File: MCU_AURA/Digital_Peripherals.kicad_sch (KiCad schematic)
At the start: 20 parts, among them J1 TF-CARD_H1.8, Q300 BSS138, Q301 BSS138, Q302 BSS138, U300 ICM-20948, U301 BMP280

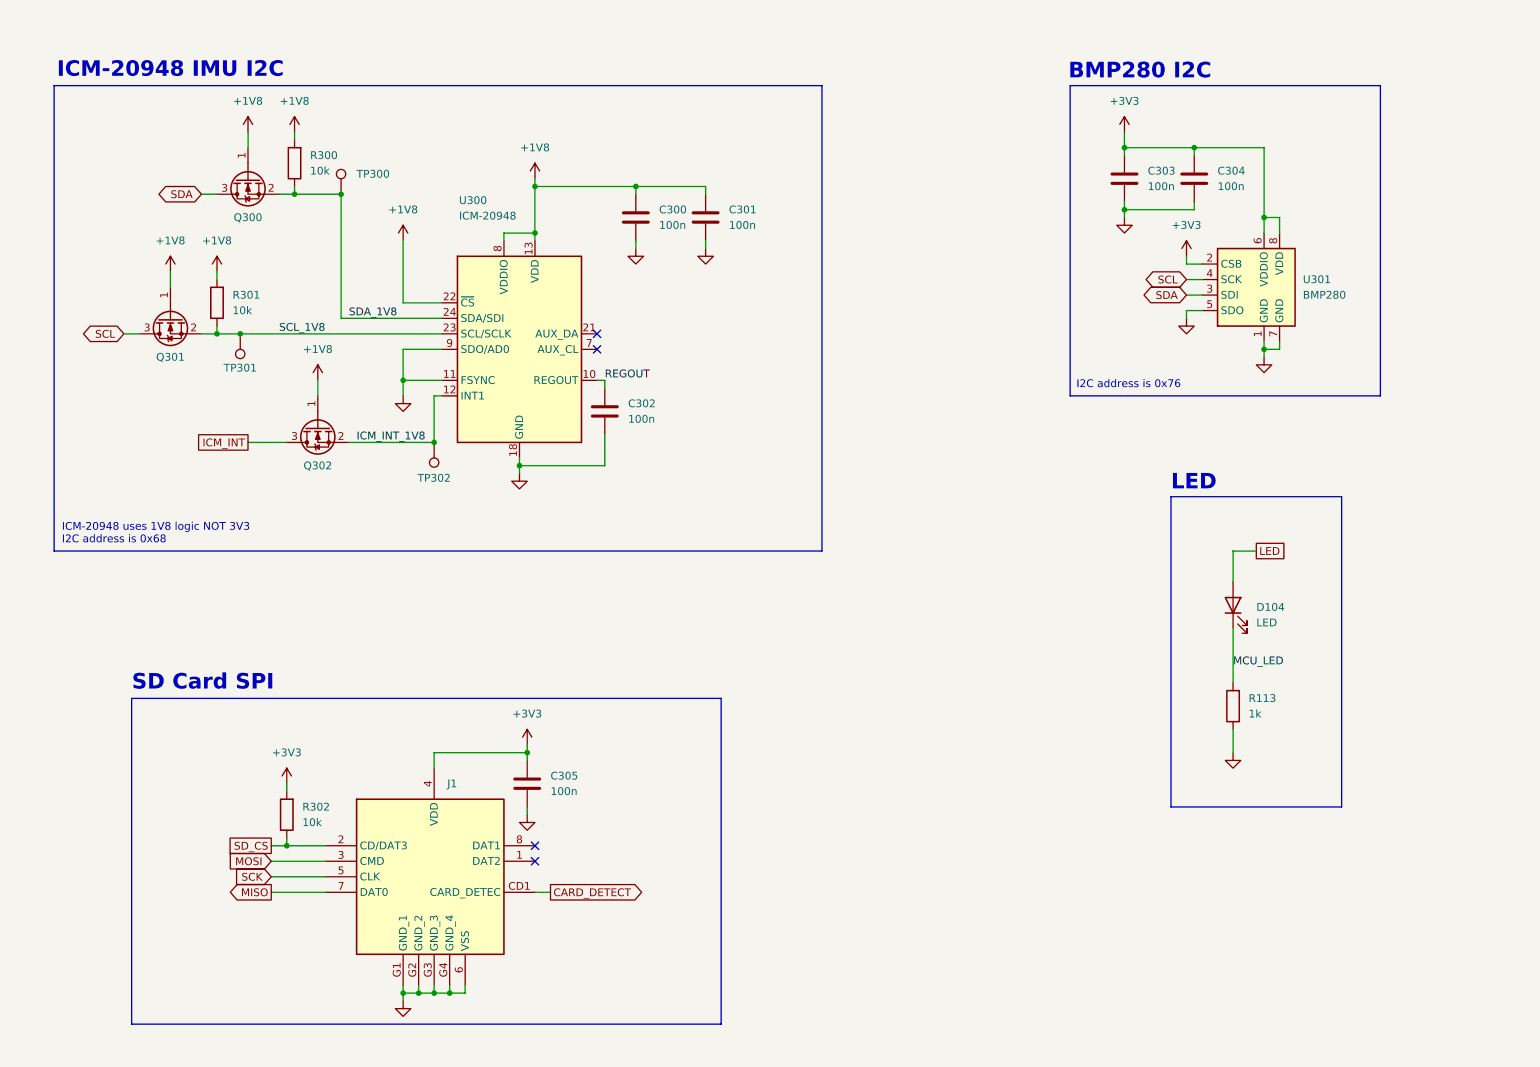
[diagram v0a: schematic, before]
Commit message: Initial Schematic Draft
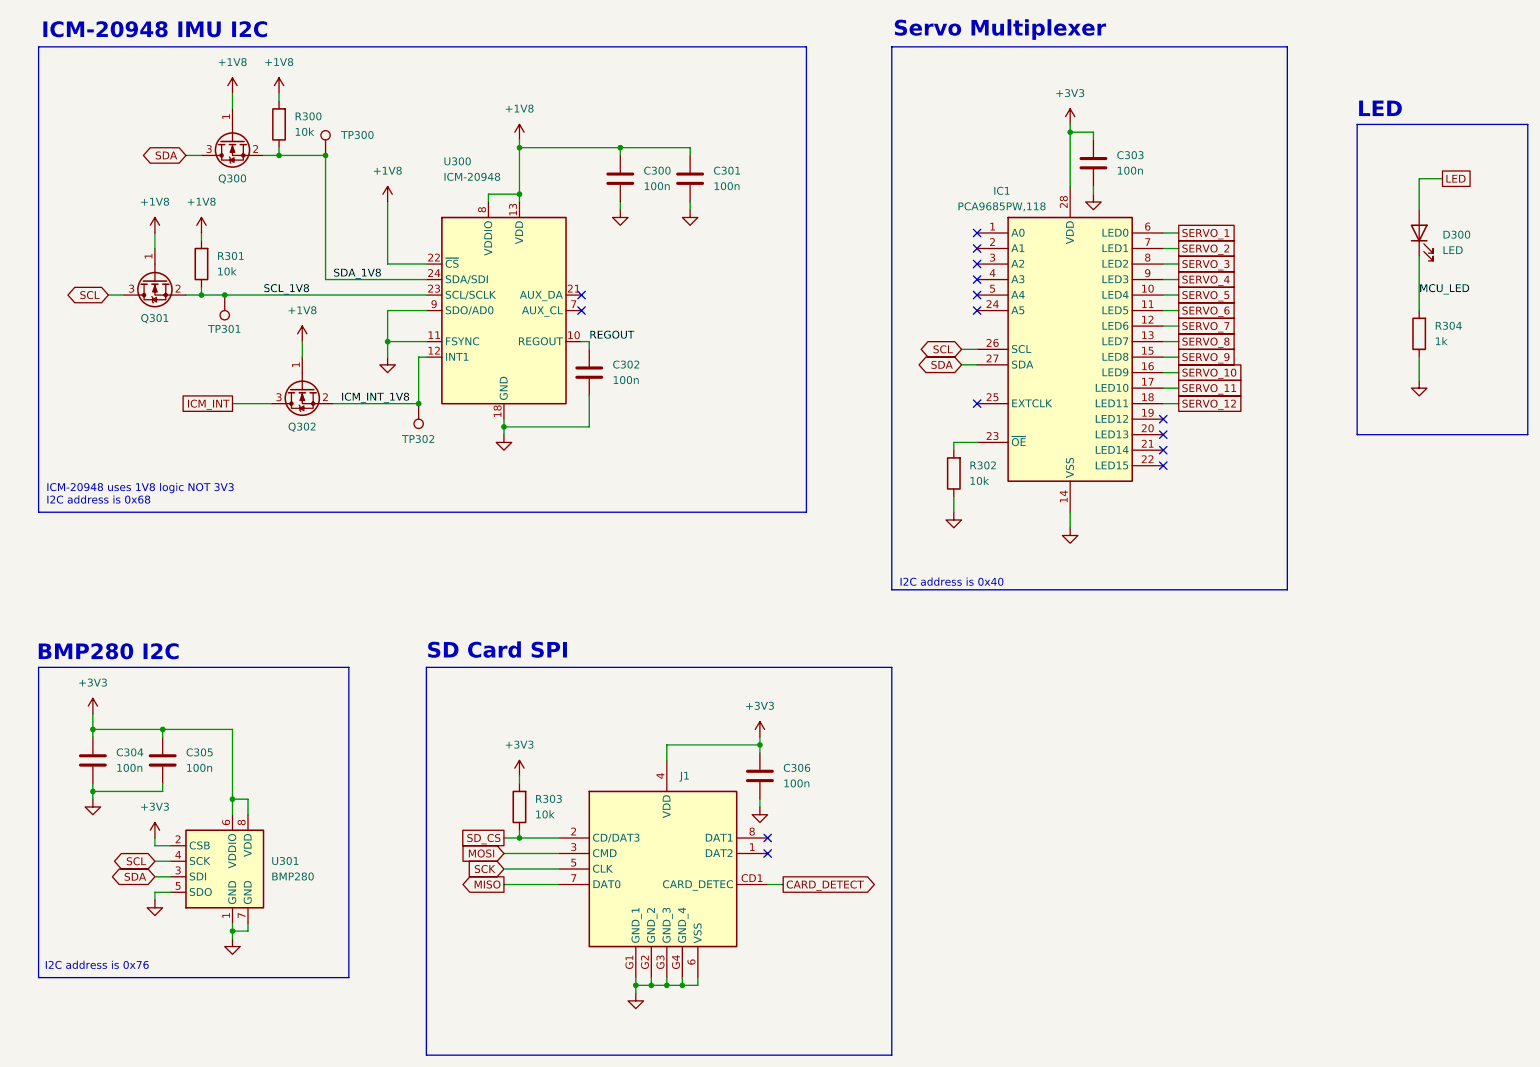
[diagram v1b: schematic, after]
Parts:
- added C303: 100n, Capacitor_SMD:C_0402_1005Metric, symbol Device:C
- added IC1: PCA9685PW,118, PCA9685PW_118:SOP65P640X110-28N, symbol PCA9685PW_118:PCA9685PW,118
- added R302: 10k, Resistor_SMD:R_0402_1005Metric, symbol Device:R
- renumbered C303 to C304, C304 to C305, C305 to C306, D104 to D300, R302 to R303, R113 to R304
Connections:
- net +3V3: now also C303.1, IC1.28 (VDD)
- net GND: now also C303.2, IC1.14 (VSS), R302.1
- net SCL: now also IC1.26 (SCL)
- net SDA: now also IC1.27 (SDA)
- new net: IC1.23 (~{OE}), R302.2
- new net SERVO_1: IC1.6 (LED0)
- new net SERVO_10: IC1.16 (LED9)
- new net SERVO_11: IC1.17 (LED10)
- new net SERVO_12: IC1.18 (LED11)
- new net SERVO_2: IC1.7 (LED1)
- new net SERVO_3: IC1.8 (LED2)
- new net SERVO_4: IC1.9 (LED3)
- new net SERVO_5: IC1.10 (LED4)
- new net SERVO_6: IC1.11 (LED5)
- new net SERVO_7: IC1.12 (LED6)
- new net SERVO_8: IC1.13 (LED7)
- new net SERVO_9: IC1.15 (LED8)
- no-connect marks 4 -> 15
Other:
- note added: "I2C address is 0x40"
- note added: "Servo Multiplexer"
- moved on the sheet: C300, C301, C302, C304, C305, C306, D300, J1, Q300, Q301, Q302, R300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
